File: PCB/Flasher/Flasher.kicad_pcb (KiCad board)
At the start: 2 copper layers, 70 x 70 mm, 62 parts, among them J1 Reset, J2 RJ12, J3 USB, J4 USB-C-Socket-V, J5 TF_PUSH, SW1 SW_Push_DPDT, U1 ESP32-S3-MINI-1-N4R2, U2 TPS562246, U3 FT231XQ, U4 TPS22916CNYFPR, U5 TPS22916CNYFPR

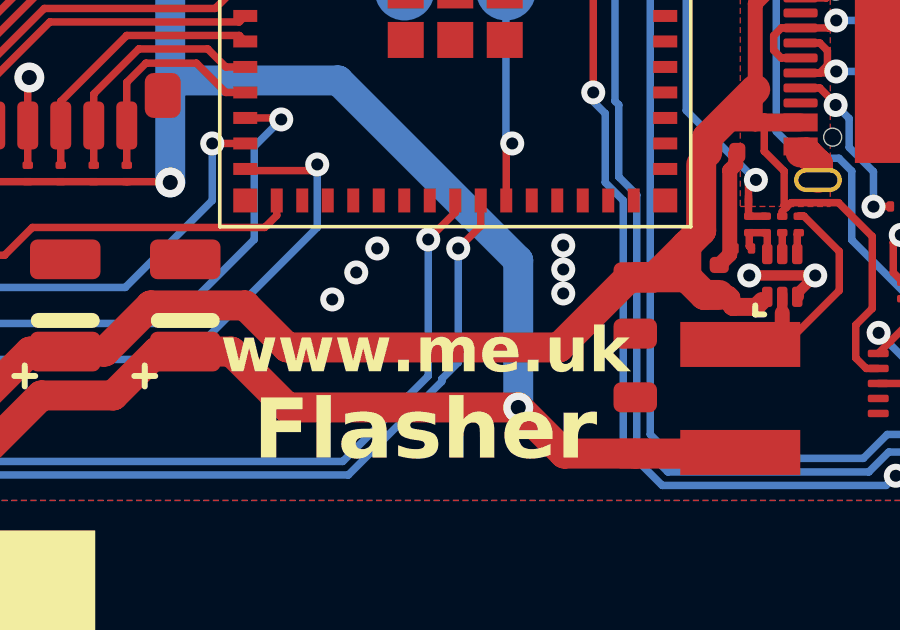
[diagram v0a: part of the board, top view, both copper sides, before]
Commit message: Library update
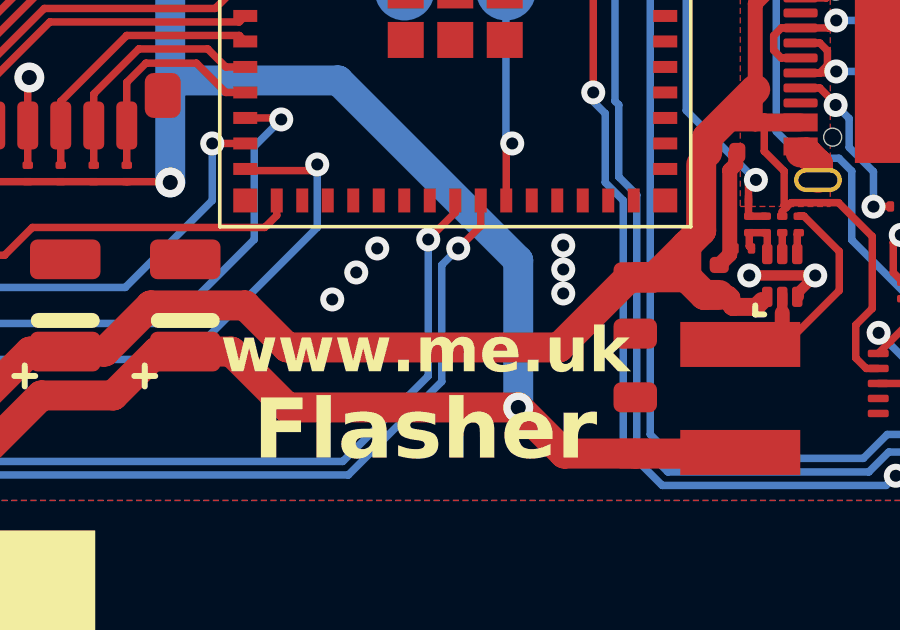
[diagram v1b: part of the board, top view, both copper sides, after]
